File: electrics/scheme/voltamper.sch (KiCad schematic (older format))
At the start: 28 parts

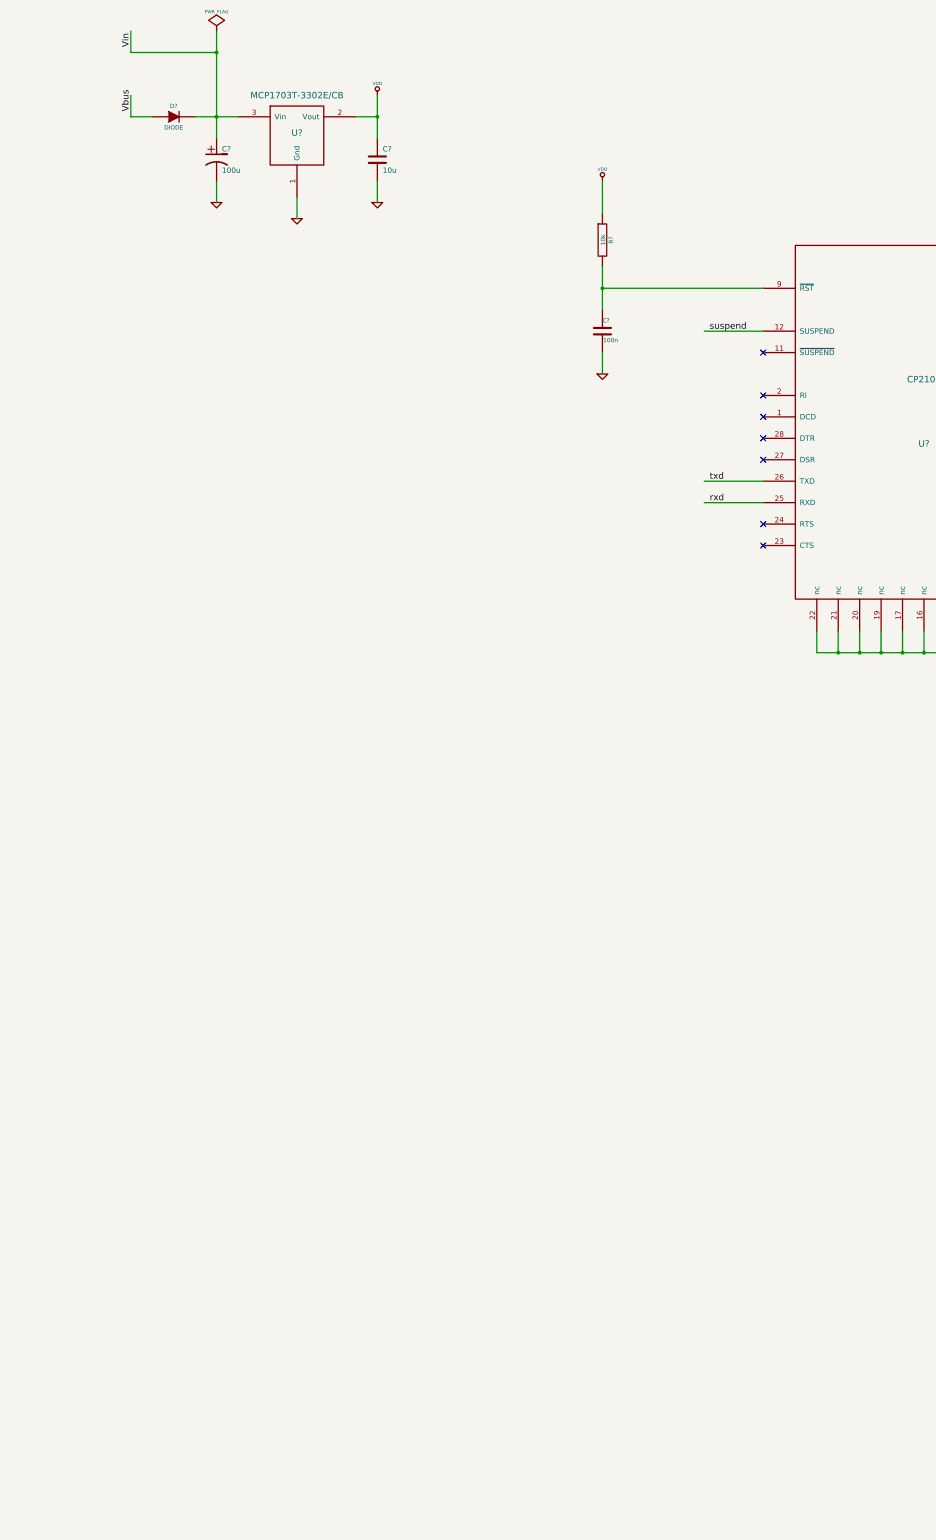
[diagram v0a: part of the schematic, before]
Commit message: a
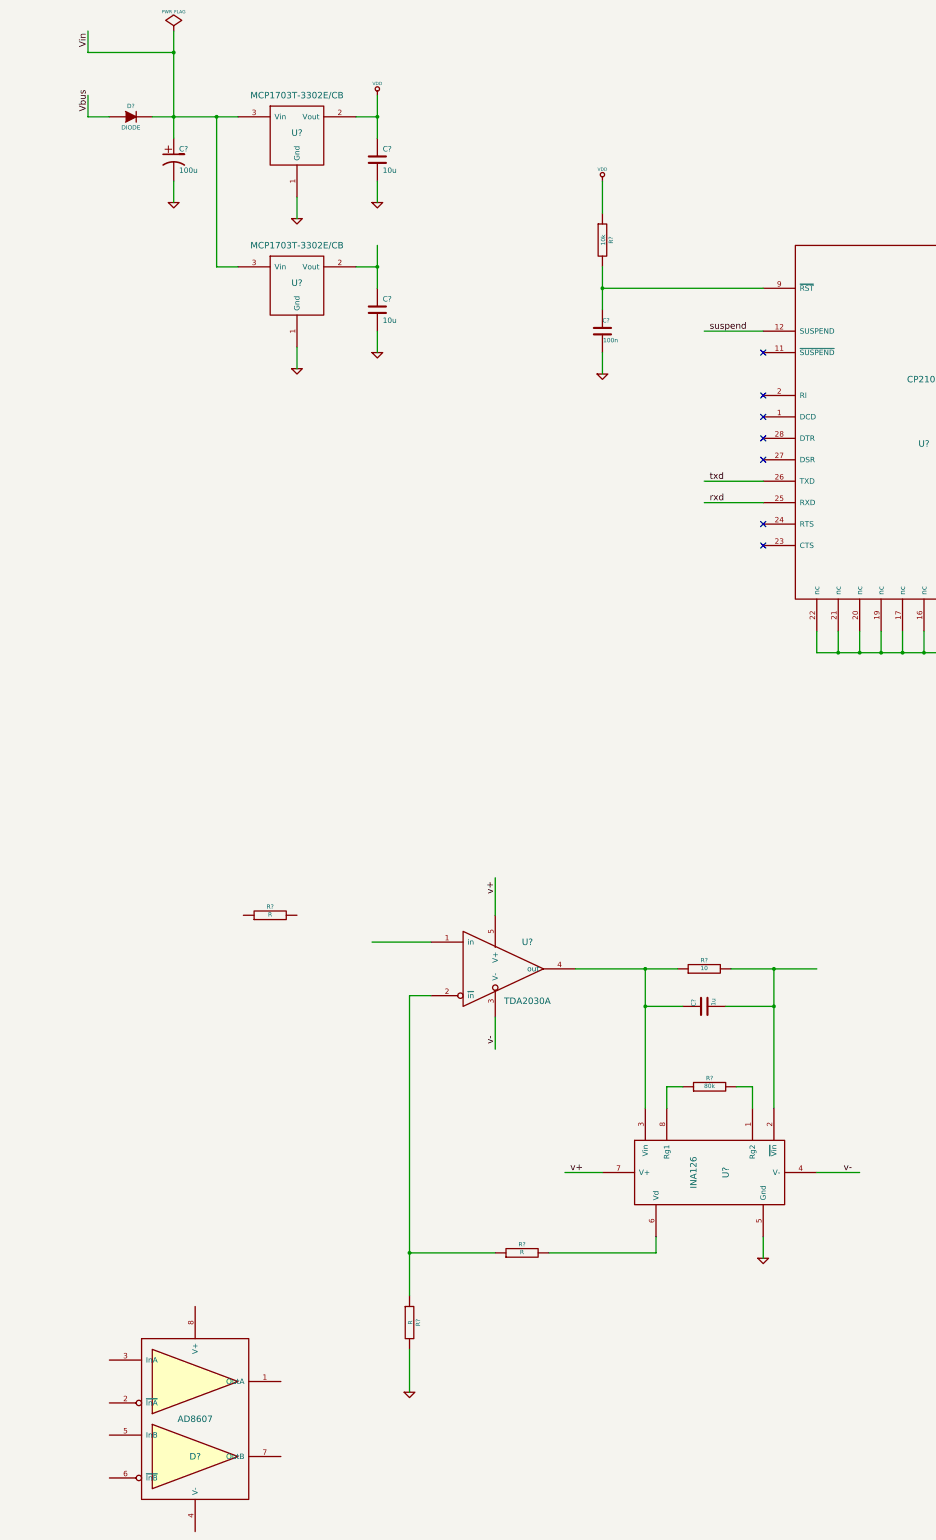
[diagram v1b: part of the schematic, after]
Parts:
- added C?: 1u, ~, symbol C
- added C?: 10u, symbol C
- added D?: AD8607, symbol AD8607
- added R?: 10, ~, symbol R
- added R?: 80k, ~, symbol R
- added R? (x3): R, ~, symbol R
- added U?: INA126, symbol INA126
- added U?: TDA2030A, ~, symbol TDA2030A
- added U?: MCP1703T-3302E/CB, ~, symbol MCP1703T-3302E/CB
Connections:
- net labels added: v+, v-
- wire segments 114 -> 142
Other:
- moved on the sheet: C?, D?
